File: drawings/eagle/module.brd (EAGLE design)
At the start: 60.6 x 80 mm, 25 parts, among them T1 2N3904, T2 2N3904

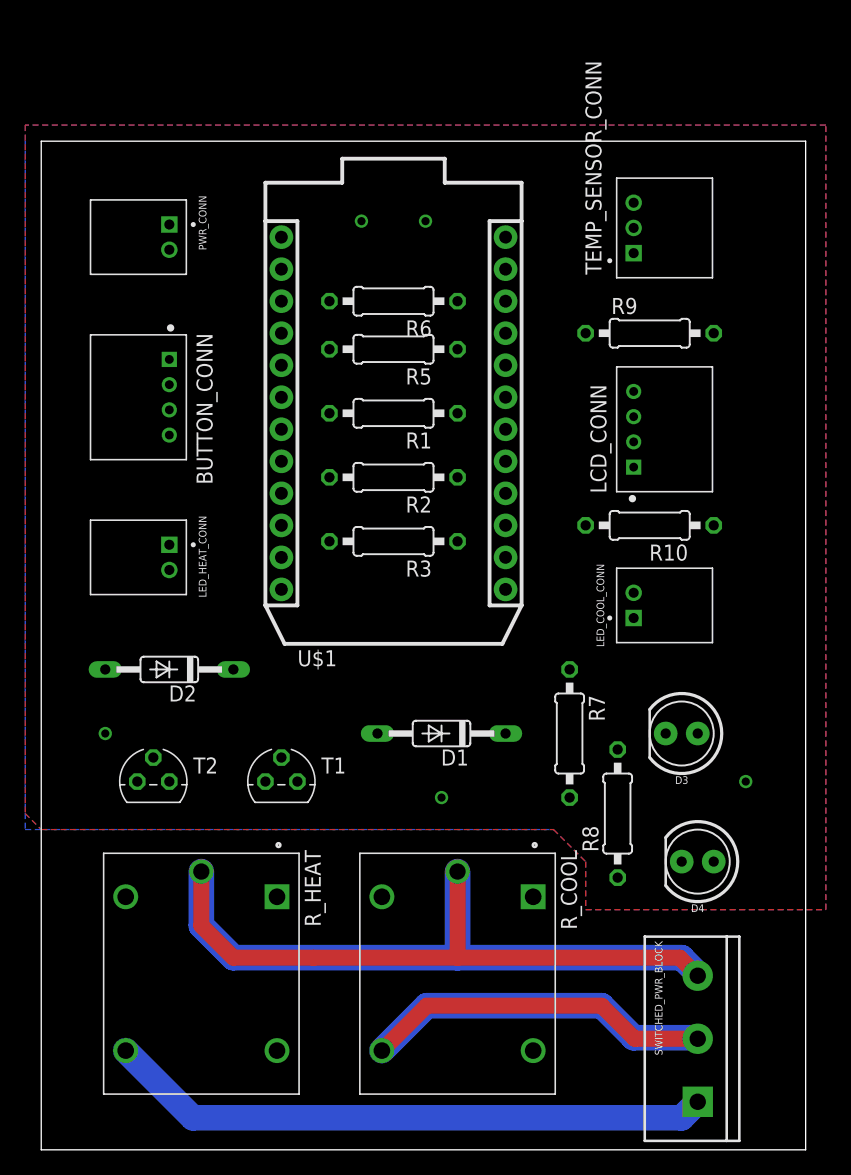
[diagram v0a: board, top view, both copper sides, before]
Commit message: Finished rev1 of the circuit board and moved to a drawings directory
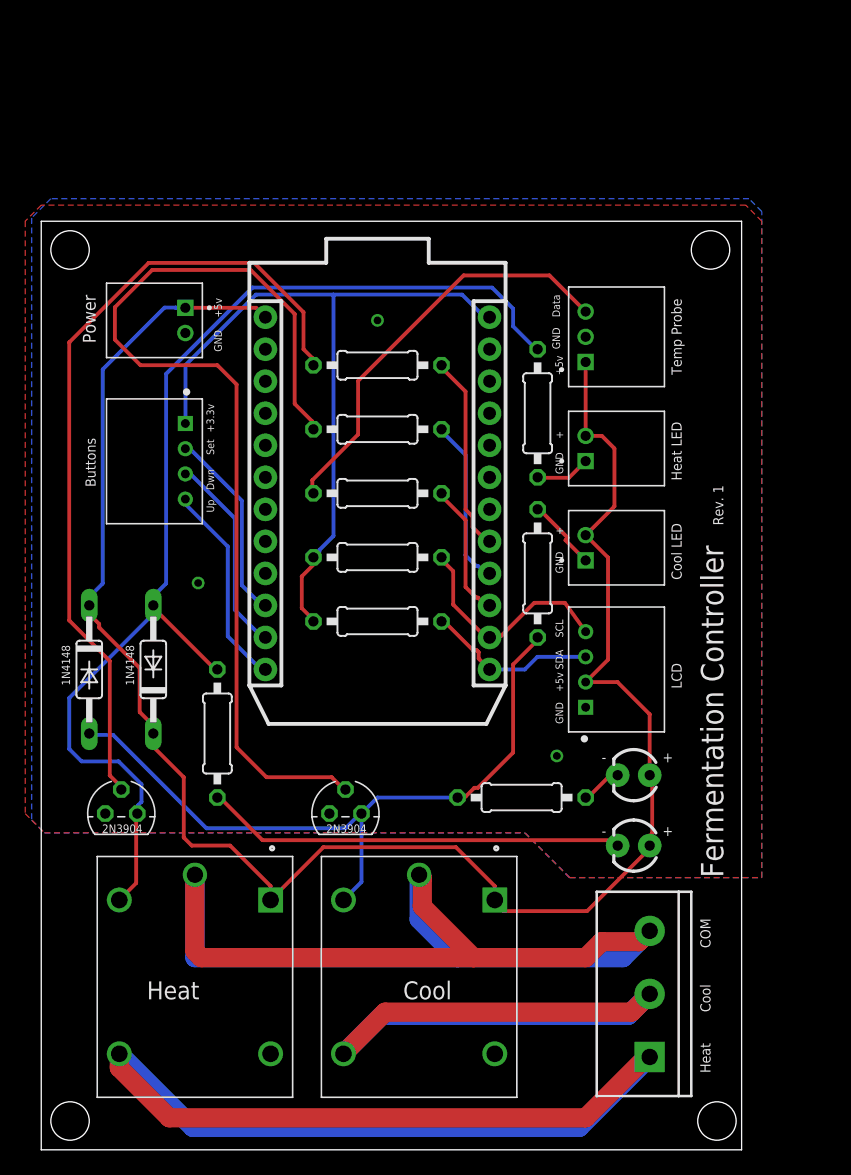
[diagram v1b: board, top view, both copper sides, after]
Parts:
- D3: value (none) -> blue; device SparkFun-LED:LED_5MM -> SparkFun-LED:LED_3MM
- D4: value (none) -> red; device SparkFun-LED:LED_5MM -> SparkFun-LED:LED_3MM
- moved LED_HEAT_CONN 34.1 mm to (43.2, 55.6), turned to 90 degrees
- moved R8 32.4 mm to (14.0, 33.0)
- moved D1 28.4 mm to (3.81, 38.1), turned to 270 degrees
- moved R9 21.0 mm to (39.4, 45.7), turned to 270 degrees
- moved LCD_CONN 19.4 mm to (43.2, 38.1)
- moved R10 12.6 mm to (39.4, 58.4), turned to 90 degrees
- moved R2 11.5 mm to (26.7, 41.9)
- moved R1 11.5 mm to (26.7, 47.0)
- moved TEMP_SENSOR_CONN 9.44 mm to (43.2, 62.5)
- moved PWR_CONN 6.73 mm to (11.4, 65.8)
- moved R5 6.48 mm to (26.7, 57.1)
- moved U$1 6.48 mm to (16.5, 33.0)
- moved R7 6.35 mm to (38.1, 27.9), turned to 180 degrees
- moved LED_COOL_CONN 5.95 mm to (43.2, 47.8)
- moved T1 5.68 mm to (24.1, 26.7)
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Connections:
- removed net BTN_DOWN: U$1.18
- removed net BTN_UP: U$1.19
- net BTN_SET: no longer U$1.20
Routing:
- net +5V: track 0.00 -> 148.8 mm
- net N$9: track 0.00 -> 92.3 mm
- net N$6: track 0.00 -> 79.2 mm
- net N$8: track 0.00 -> 64.6 mm
- net +3V3: track 0.00 -> 59.2 mm
- net N$4: track 0.00 -> 56.6 mm
- net RLY_HEAT: track 48.1 -> 93.6 mm
- net N$13: track 0.00 -> 33.3 mm
- net TEMP_DATA: track 0.00 -> 33.2 mm
- net SCL: track 0.00 -> 18.0 mm
- net BTN_COOL: track 0.00 -> 16.4 mm
- net BTN_HEAT: track 0.00 -> 16.0 mm
- net HEAT_CTRL: track 0.00 -> 15.8 mm
- net BTN_SET: track 0.00 -> 15.5 mm
- net SDA: track 0.00 -> 13.7 mm
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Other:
- board size 60.6 x 80 mm -> 55.5 x 73.7 mm
- board text added: "+"
- board text added: "+3.3v"
- board text added: "+5v"
- board text added: "-"
- board text added: "1N4148"
- board text added: "2N3904"
- board text added: "Buttons"
- board text added: "COM"
- board text added: "Cool"
- board text added: "Cool LED"
- board text added: "Data"
- board text added: "Dwn"
- board text added: "Fermentation Controller"
- board text added: "GND"
- board text added: "Heat"
- board text added: "Heat LED"
- board text added: "LCD"
- board text added: "Power"
- board text added: "Rev. 1"
- board text added: "SCL"
- board text added: "SDA"
- board text added: "Set"
- board text added: "Temp Probe"
- board text added: "Up"
